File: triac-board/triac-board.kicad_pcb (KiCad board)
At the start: 2 copper layers, 100 x 80 mm, 75 parts, among them J1 Screw_Terminal_01x02, J10 Screw_Terminal_01x02, J11 Screw_Terminal_01x02, J12 Screw_Terminal_01x02, J13 Screw_Terminal_01x02, J14 Screw_Terminal_01x02, J15 Screw_Terminal_01x02, J16 Screw_Terminal_01x02, J17 Screw_Terminal_01x02, J18 Screw_Terminal_01x02, J19 Screw_Terminal_01x02, J2 Screw_Terminal_01x02, J20 Conn_01x01_Male, J21 Conn_01x01_Male, J3 Screw_Terminal_01x02, J4 Screw_Terminal_01x02, J5 Screw_Terminal_01x02, J6 Screw_Terminal_01x02, J7 Screw_Terminal_01x02, J8 Screw_Terminal_01x02, J9 Screw_Terminal_01x02, Q1 BTA16-600BW, Q10 BTA16-600BW, Q2 BTA16600BW, Q3 BTA16-600BW, Q4 BTA16-600BW, Q5 BTA16-600BW, Q6 BTA16-600BW, Q7 BTA16-600BW, Q8 BTA16-600BW, Q9 BTA16-600BW, U1 MOC3063M, U10 MOC3063M, U2 MOC3063M, U3 MOC3063M, U4 MOC3063M, U5 MOC3063M, U6 MOC3063M, U7 MOC3063M, U8 MOC3063M, U9 MOC3063M

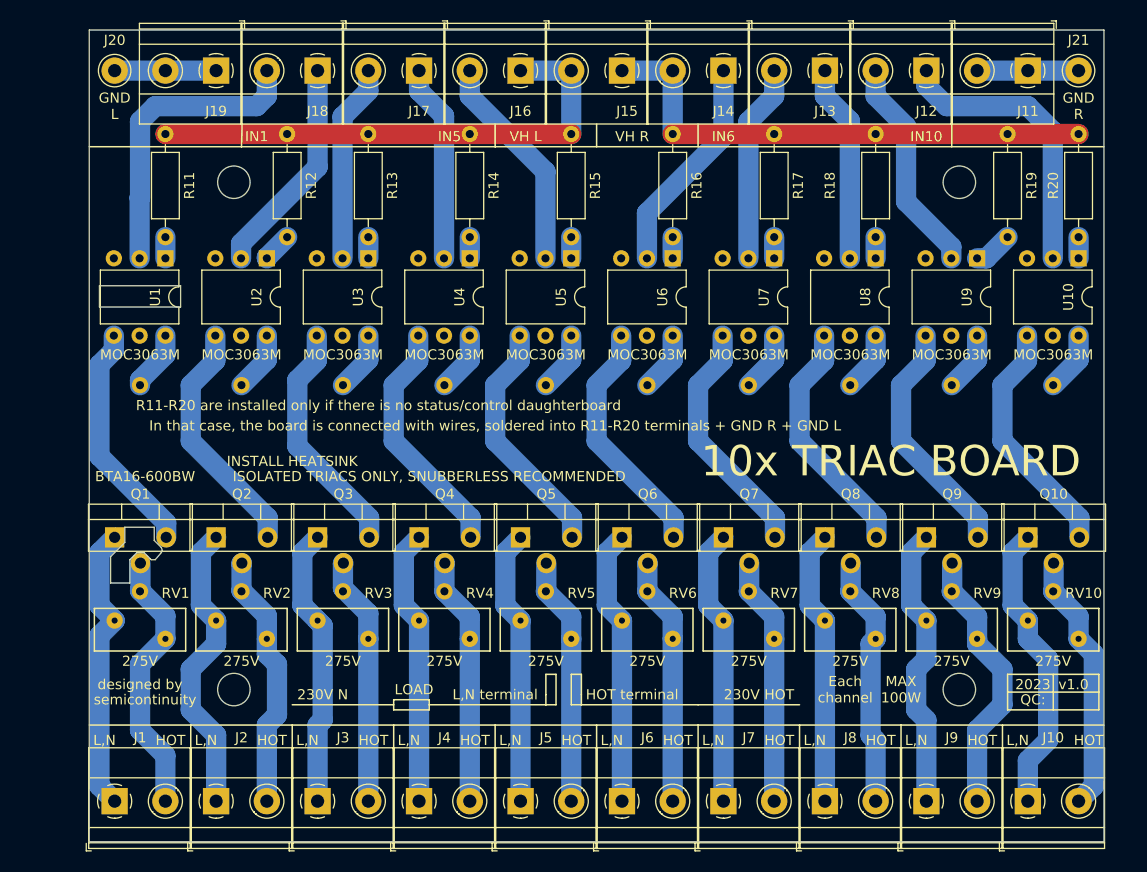
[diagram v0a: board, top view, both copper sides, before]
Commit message: triac-board
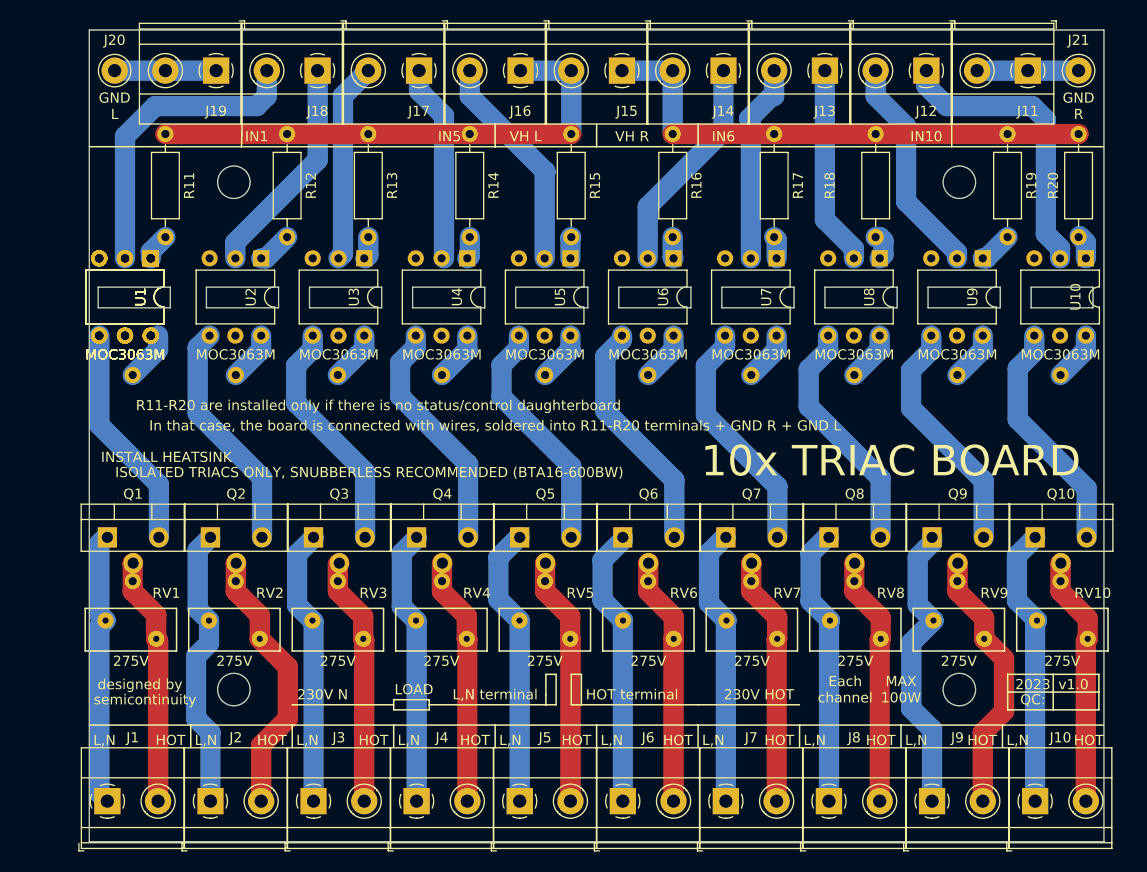
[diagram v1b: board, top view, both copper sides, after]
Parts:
- added U1 (x3): MOC3063M, Package_DIP:DIP-6_W7.62mm, F.Cu at (156.1, 82.5)
- moved U1 1.44 mm to (156.1, 82.5)
- moved R1 1.23 mm to (154.3, 94.0)
- moved R10 1.23 mm to (245.7, 94.0)
- moved R2 1.15 mm to (164.4, 94.0)
- moved R9 1.15 mm to (235.6, 94.0)
- moved R3 1.12 mm to (174.5, 94.0)
- moved R8 1.08 mm to (225.4, 94.0)
- moved R4 1.03 mm to (184.8, 94.0)
- moved R7 1.03 mm to (215.2, 94.0)
- moved R5 1.00 mm to (194.9, 94.0)
- moved R6 1.00 mm to (205.1, 94.0)
- moved RV1 0.90 mm to (156.6, 120.0)
- moved RV10 0.90 mm to (248.4, 120.0)
- moved J1 0.72 mm to (151.8, 136.0)
- moved J10 0.72 mm to (243.2, 136.0)
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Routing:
- net Net-(J1-Pad2): track 26.6 -> 24.5 mm
- net Net-(J1-Pad1): track 28.5 -> 27.1 mm
- net Net-(J2-Pad2): track 25.3 -> 26.7 mm
- net Net-(J10-Pad1): track 28.9 -> 27.6 mm
- net Net-(J2-Pad1): track 29.3 -> 28.1 mm
- net Net-(J10-Pad2): track 25.8 -> 24.7 mm
- net Net-(Q2-Pad3): track 24.0 -> 23.0 mm
- net Net-(R9-Pad1): track 5.92 -> 4.92 mm
- net Net-(R8-Pad1): track 5.92 -> 4.92 mm
- net Net-(R7-Pad1): track 5.92 -> 4.92 mm
- net Net-(R6-Pad1): track 5.92 -> 4.92 mm
- net Net-(R5-Pad1): track 5.92 -> 4.92 mm
- net Net-(R4-Pad1): track 5.92 -> 4.92 mm
- net Net-(R2-Pad1): track 5.92 -> 4.92 mm
- net Net-(R10-Pad1): track 5.92 -> 4.92 mm
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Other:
- outline, holes or cut-outs redrawn
- board text added: "5.00"
- board text added: "5.08"
- board text added: "ISOLATED TRIACS ONLY, SNUBBERLESS RECOMMENDED (BTA16-600BW)"
- board text removed: "ISOLATED TRIACS ONLY, SNUBBERLESS RECOMMENDED"
